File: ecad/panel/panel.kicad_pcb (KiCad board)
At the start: 4 copper layers, 165.5 x 51.6 mm, 204 parts, among them J2 Conn_01x03_Pin, J3 USB4105-GF-A, J4 5017868090, SW1 SW_SPDT, SW10 SW_SPDT, SW11 SW_SPDT, SW12 SW_SPDT, SW13 SW_SPDT, SW14 SW_SPDT, SW15 SW_SPDT, SW16 SW_SPDT, SW17 SW_Push, SW18 SW_Push, SW19 SW_Push, SW2 SW_SPDT, SW20 SW_Push, SW21 SW_Push, SW22 SW_Push, SW23 SW_Push, SW24 SW_Push, SW25 SW_Push, SW26 SW_Push, SW27 SW_Push, SW28 SW_Push, SW29 SW_Push, SW3 SW_SPDT, SW30 SW_Push, SW4 SW_SPDT, SW5 SW_SPDT, SW6 SW_SPDT, SW7 SW_SPDT, SW8 SW_SPDT, SW9 SW_SPDT, U1 TLC59211IN, U10 NCP1117-3.3_SOT223, U2 TLC59211IN, U3 TLC59211IN, U4 TLC59211IN, U5 TLC59211IN, U6 RP2350_80QFN, U7 W25Q128JVS, U8 MCP23017_SO, U9 MCP23017_SO, X1 ABM8-272-T3

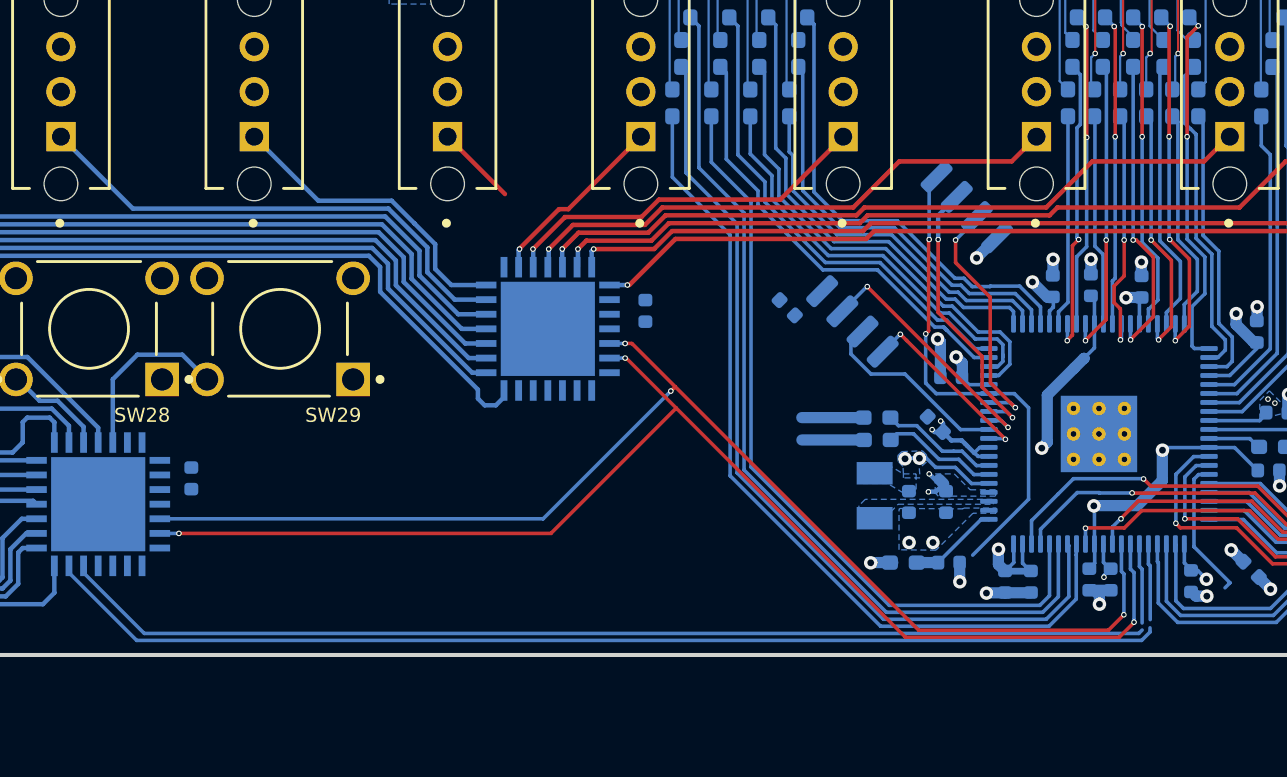
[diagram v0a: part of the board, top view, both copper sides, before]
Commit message: minor panel adj.
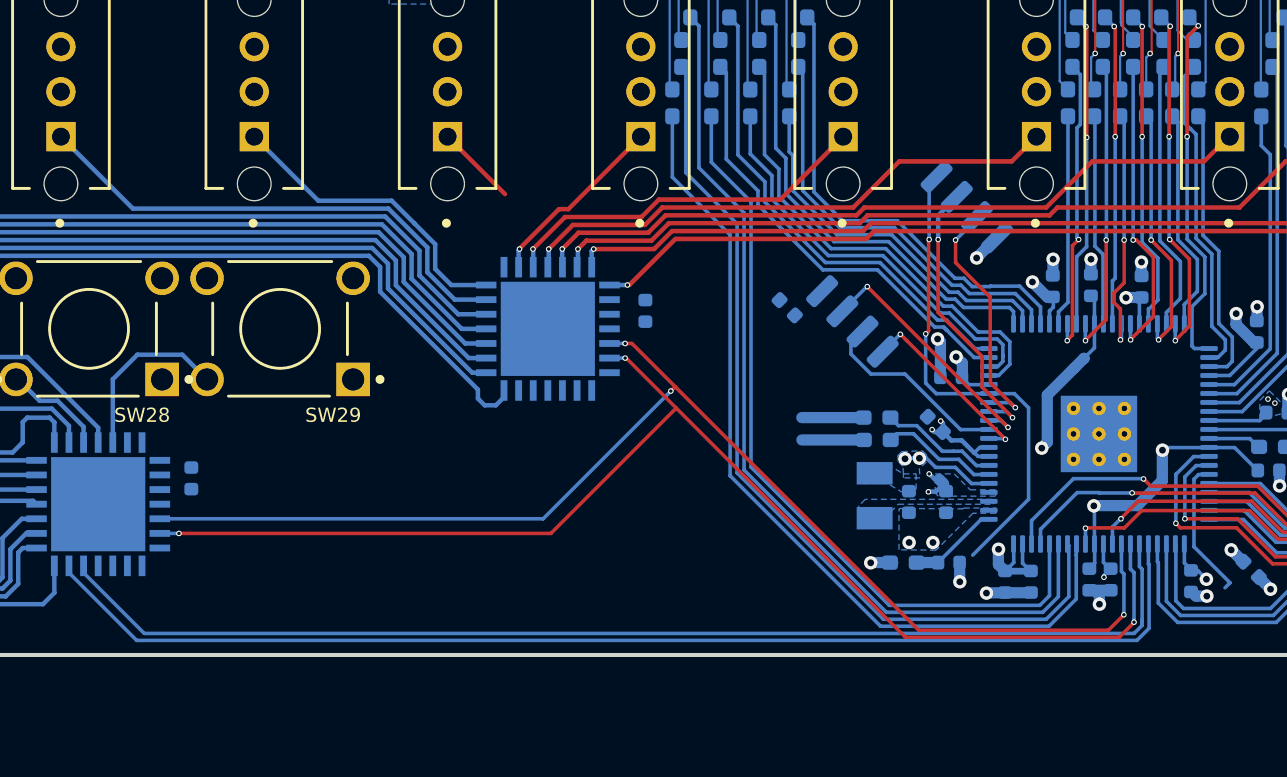
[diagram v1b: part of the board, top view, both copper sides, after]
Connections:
- U6 pad 45: unconnected-(U6-GPIO36-Pad45) -> /PUSH_INTA
- U6 pad 46: unconnected-(U6-GPIO37-Pad46) -> /PUSH_INTB
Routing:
- net /PUSH_INTB: track 48.6 -> 52.5 mm
- net /PUSH_INTA: track 50.0 -> 53.6 mm
- net unconnected-(U6-GPIO37-Pad46): track 3.56 -> 0.00 mm
- net unconnected-(U6-GPIO36-Pad45): track 3.39 -> 0.00 mm
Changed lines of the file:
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@@
 	(net 250 "GND")
 	(net 251 "/BUS24")
-	(net 252 "unconnected-(U6-GPIO36-Pad45)")
-	(net 253 "unconnected-(U6-GPIO37-Pad46)")
-	(net 254 "unconnected-(D37-K-Pad1)")
-	(net 255 "SINGLE_STEP")
-	(net 256 "/M1_LED")
-	(net 257 "unconnected-(U8-GPB7-Pad8)")
-	(net 258 "/PUSH_INTA")
-	(net 259 "/PUSH_INTB")
-	(net 260 "unconnected-(U8-GPB6-Pad7)")
-	(net 261 "unconnected-(U8-GPB5-Pad6)")
+	(net 252 "unconnected-(D37-K-Pad1)")
+	(net 253 "SINGLE_STEP")
+	(net 254 "/M1_LED")
+	(net 255 "unconnected-(U8-GPB7-Pad8)")
+	(net 256 "/PUSH_INTA")
+	(net 257 "/PUSH_INTB")
+	(net 258 "unconnected-(U8-GPB6-Pad7)")
+	(net 259 "unconnected-(U8-GPB5-Pad6)")
 	(footprint "Diode_SMD:D_0402_1005Metric_Pad0.77x0.64mm_HandSolder"
 		(layer "F.Cu")
@@
 			(layers "F.Cu" "F.Paste" "F.Mask")
 			(roundrect_rratio 0.25)
-			(net 254 "unconnected-(D37-K-Pad1)")
+			(net 252 "unconnected-(D37-K-Pad1)")
 			(pinfunction "K")
 			(pintype "passive")
@@
 			(layers "*.Cu" "*.Mask")
 			(remove_unused_layers no)
-			(net 255 "SINGLE_STEP")
+			(net 253 "SINGLE_STEP")
 			(pinfunction "2")
 			(pintype "passive")
@@
 			(size 1.78 0.42)
 			(layers "B.Cu" "B.Paste" "B.Mask")
-			(net 256 "/M1_LED")
+			(net 254 "/M1_LED")
 			(pinfunction "*Y4")
 			(pintype "output")
@@
 			(size 1.4 2.6)
 			(layers "B.Cu" "B.Paste" "B.Mask")
-			(net 256 "/M1_LED")
+			(net 254 "/M1_LED")
 			(pinfunction "K")
 			(pintype "passive")
@@
 			(layers "B.Cu" "B.Paste" "B.Mask")
 			(roundrect_rratio 0.25)
-			(net 252 "unconnected-(U6-GPIO36-Pad45)")
+			(net 256 "/PUSH_INTA")
 			(pinfunction "GPIO36")
 			(pintype "bidirectional")
@@
 			(layers "B.Cu" "B.Paste" "B.Mask")
 			(roundrect_rratio 0.25)
-			(net 253 "unconnected-(U6-GPIO37-Pad46)")
+			(net 257 "/PUSH_INTB")
 			(pinfunction "GPIO37")
 			(pintype "bidirectional")
@@
 			(size 0.3048 0.9144)
 			(layers "B.Cu" "B.Paste" "B.Mask")
-			(net 261 "unconnected-(U8-GPB5-Pad6)")
+			(net 259 "unconnected-(U8-GPB5-Pad6)")
 			(pinfunction "GPB5")
 			(pintype "bidirectional+no_connect")
@@
 			(size 0.3048 0.9144)
 			(layers "B.Cu" "B.Paste" "B.Mask")
-			(net 260 "unconnected-(U8-GPB6-Pad7)")
+			(net 258 "unconnected-(U8-GPB6-Pad7)")
 			(pinfunction "GPB6")
 			(pintype "bidirectional+no_connect")
@@
 			(size 0.3048 0.9144)
 			(layers "B.Cu" "B.Paste" "B.Mask")
-			(net 257 "unconnected-(U8-GPB7-Pad8)")
+			(net 255 "unconnected-(U8-GPB7-Pad8)")
 			(pinfunction "GPB7")
 			(pintype "bidirectional+no_connect")
@@
 			(size 0.3048 0.9144)
 			(layers "B.Cu" "B.Paste" "B.Mask")
-			(net 259 "/PUSH_INTB")
+			(net 257 "/PUSH_INTB")
 			(pinfunction "INTB")
 			(pintype "tri_state")
@@
 			(size 0.3048 0.9144)
 			(layers "B.Cu" "B.Paste" "B.Mask")
-			(net 258 "/PUSH_INTA")
+			(net 256 "/PUSH_INTA")
 			(pinfunction "INTA")
 			(pintype "tri_state")
@@
 			(size 0.3048 0.9144)
 			(layers "B.Cu" "B.Paste" "B.Mask")
-			(net 255 "SINGLE_STEP")
+			(net 253 "SINGLE_STEP")
 			(pinfunction "GPA2")
 			(pintype "bidirectional")
@@
 	)
 	(segment
-		(start 156.177319 60.737157)
-		(end 156.177319 58.822681)
-		(width 0.16)
-		(layer "B.Cu")
-		(net 15)
-	)
-	(segment
 		(start 156.3 58.7)
-		(end 156.3 52.5)
+		(end 156.3 52.4)
 		(width 0.16)
 		(layer "B.Cu")
@@
 	)
 	(segment
-		(start 156.177319 58.822681)
-		(end 156.3 58.7)
+		(start 156.177319 60.737157)
+		(end 156.177319 58.822681)
 		(width 0.16)
 		(layer "B.Cu")
@@
 	)
 	(segment
-		(start 156.3 52.5)
-		(end 156.3 52.4)
+		(start 156.177319 58.822681)
+		(end 156.3 58.7)
 		(width 0.16)
 		(layer "B.Cu")
@@
 	)
 	(segment
-		(start 156.7 58.6)
-		(end 156.254112 59.045888)
+		(start 156.254112 59.784768)
+		(end 156.530872 60.061528)
 		(width 0.16)
 		(layer "F.Cu")
@@
 	(segment
 		(start 156.7 57)
-		(end 156.7 58.6)
+		(end 156.7 58.9)
 		(width 0.16)
 		(layer "F.Cu")
@@
 	)
 	(segment
-		(start 156.254112 59.784768)
-		(end 156.530872 60.061528)
+		(start 156.7 58.9)
+		(end 156.254112 59.345888)
 		(width 0.16)
 		(layer "F.Cu")
@@
 	)
 	(segment
-		(start 156.530872 60.061528)
-		(end 156.530872 61.427412)
+		(start 156.254112 59.345888)
+		(end 156.254112 59.784768)
 		(width 0.16)
 		(layer "F.Cu")
@@
 	)
 	(segment
-		(start 156.254112 59.045888)
-		(end 156.254112 59.784768)
+		(start 156.530872 60.061528)
+		(end 156.530872 61.427412)
 		(width 0.16)
 		(layer "F.Cu")
@@
 	)
 	(segment
-		(start 157.858754 71.493214)
-		(end 157.858754 73.885155)
-		(width 0.16)
-		(layer "B.Cu")
-		(net 252)
-	)
-	(segment
-		(start 157.778753 70.528722)
-		(end 157.778753 71.413212)
-		(width 0.16)
-		(layer "B.Cu")
-		(net 252)
-	)
-	(segment
-		(start 157.778753 71.413212)
-		(end 157.858754 71.493214)
-		(width 0.16)
-		(layer "B.Cu")
-		(net 252)
-	)
-	(segment
-		(start 157.378753 71.522329)
-		(end 157.498754 71.64233)
-		(width 0.16)
-		(layer "B.Cu")
-		(net 253)
-	)
-	(segment
-		(start 157.498754 71.64233)
-		(end 157.498754 74.034272)
-		(width 0.16)
-		(layer "B.Cu")
-		(net 253)
-	)
-	(segment
-		(start 157.378753 70.528723)
-		(end 157.378753 71.522329)
-		(width 0.16)
-		(layer "B.Cu")
-		(net 253)
-	)
-	(segment
 		(start 106.800001 72.5)
 		(end 67.6 72.5)
 		(width 0.2)
 		(layer "B.Cu")
-		(net 255)
+		(net 253)
 	)
 	(segment
@@
 		(width 0.2)
 		(layer "B.Cu")
-		(net 255)
+		(net 253)
 	)
 	(segment
@@
 		(width 0.2)
 		(layer "B.Cu")
-		(net 255)
+		(net 253)
 	)
 	(segment
@@
 		(width 0.2)
 		(layer "B.Cu")
-		(net 255)
+		(net 253)
 	)
 	(segment
@@
 		(width 0.2)
 		(layer "B.Cu")
-		(net 255)
+		(net 253)
 	)
 	(segment
@@
 		(width 0.2)
 		(layer "B.Cu")
-		(net 255)
+		(net 253)
 	)
 	(segment
@@
 		(width 0.2)
 		(layer "B.Cu")
-		(net 255)
+		(net 253)
 	)
 	(segment
@@
 		(width 0.2)
 		(layer "B.Cu")
-		(net 255)
+		(net 253)
 	)
 	(segment
@@
 		(width 0.2)
 		(layer "B.Cu")
-		(net 256)
+		(net 254)
 	)
 	(segment
@@
 		(width 0.2)
 		(layer "B.Cu")
-		(net 256)
+		(net 254)
 	)
 	(segment
@@
 		(width 0.2)
 		(layer "B.Cu")
-		(net 256)
+		(net 254)
 	)
 	(segment
@@
 		(width 0.2)
 		(layer "B.Cu")
-		(net 256)
+		(net 254)
 	)
 	(segment
@@
 		(width 0.2)
 		(layer "B.Cu")
-		(net 256)
+		(net 254)
 	)
 	(segment
@@
 		(width 0.2)
 		(layer "B.Cu")
-		(net 256)
+		(net 254)
 	)
 	(segment
@@
 		(width 0.2)
 		(layer "B.Cu")
-		(net 256)
+		(net 254)
 	)
 	(segment
@@
 		(width 0.16)
 		(layer "B.Cu")
-		(net 258)
+		(net 256)
 	)
 	(segment
 		(start 112.768799 74.81)
-		(end 157.478406 74.81)
+		(end 157.269206 74.81)
 		(width 0.16)
 		(layer "B.Cu")
-		(net 258)
+		(net 256)
 	)
 	(segment
-		(start 157.478406 74.81)
-		(end 157.85 74.438406)
+		(start 157.778753 71.413212)
+		(end 157.778753 70.528722)
 		(width 0.16)
 		(layer "B.Cu")
-		(net 258)
+		(net 256)
+	)
+	(segment
+		(start 157.808754 74.270452)
+		(end 157.808754 71.443213)
+		(width 0.16)
+		(layer "B.Cu")
+		(net 256)
 	)
 	(segment
@@
 		(width 0.16)
 		(layer "B.Cu")
-		(net 258)
+		(net 256)
 	)
 	(segment
-		(start 157.85 74.438406)
-		(end 157.85 74.25)
+		(start 157.808754 71.443213)
+		(end 157.778753 71.413212)
 		(width 0.16)
 		(layer "B.Cu")
-		(net 258)
+		(net 256)
 	)
 	(segment
-		(start 157.35 74.5)
-		(end 157.5 74.35)
+		(start 157.269206 74.81)
+		(end 157.808754 74.270452)
 		(width 0.16)
 		(layer "B.Cu")
-		(net 259)
+		(net 256)
 	)
 	(segment
-		(start 113.1088 74.5)
-		(end 157.35 74.5)
+		(start 157.1408 74.5)
+		(end 157.498754 74.142046)
 		(width 0.16)
 		(layer "B.Cu")
-		(net 259)
+		(net 257)
 	)
 	(segment
-		(start 110.406801 71.493201)
-		(end 110.406801 71.798001)
+		(start 157.378753 71.522329)
+		(end 157.498754 71.64233)
+		(width 0.16)
+		(layer "B.Cu")
+		(net 257)
+	)
+	(segment
+		(start 113.1088 74.5)
+		(end 157.1408 74.5)
 		(width 0.16)
 		(layer "B.Cu")
-		(net 259)
+		(net 257)
 	)
 	(segment
@@
 		(width 0.16)
 		(layer "B.Cu")
-		(net 259)
+		(net 257)
+	)
+	(segment
+		(start 157.498754 71.64233)
+		(end 157.498754 74.034272)
+		(width 0.16)
+		(layer "B.Cu")
+		(net 257)
+	)
+	(segment
+		(start 157.378753 70.528723)
+		(end 157.378753 71.522329)
+		(width 0.16)
+		(layer "B.Cu")
+		(net 257)
+	)
+	(segment
+		(start 157.498754 74.142046)
+		(end 157.498754 73.9)
+		(width 0.16)
+		(layer "B.Cu")
+		(net 257)
+	)
+	(segment
+		(start 110.406801 71.493201)
+		(end 110.406801 71.798001)
+		(width 0.16)
+		(layer "B.Cu")
+		(net 257)
 	)
 	(zone
